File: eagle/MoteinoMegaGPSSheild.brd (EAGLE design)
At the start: 58.1 x 33.6 mm, 32 parts, among them J1 BilgeSwitch, J2 Button, J3 LED, J4 DS18B20, J5 DS18B20, J6 GND, J7 OKI-78SR-5/1.5, J8 5V, J9 12-24V_VCC, Q1 NDP6020P, Q2 IRF9Z14PBF, Q3 2N7000, Q4 IRF9Z14PBF, Q5 2N7000

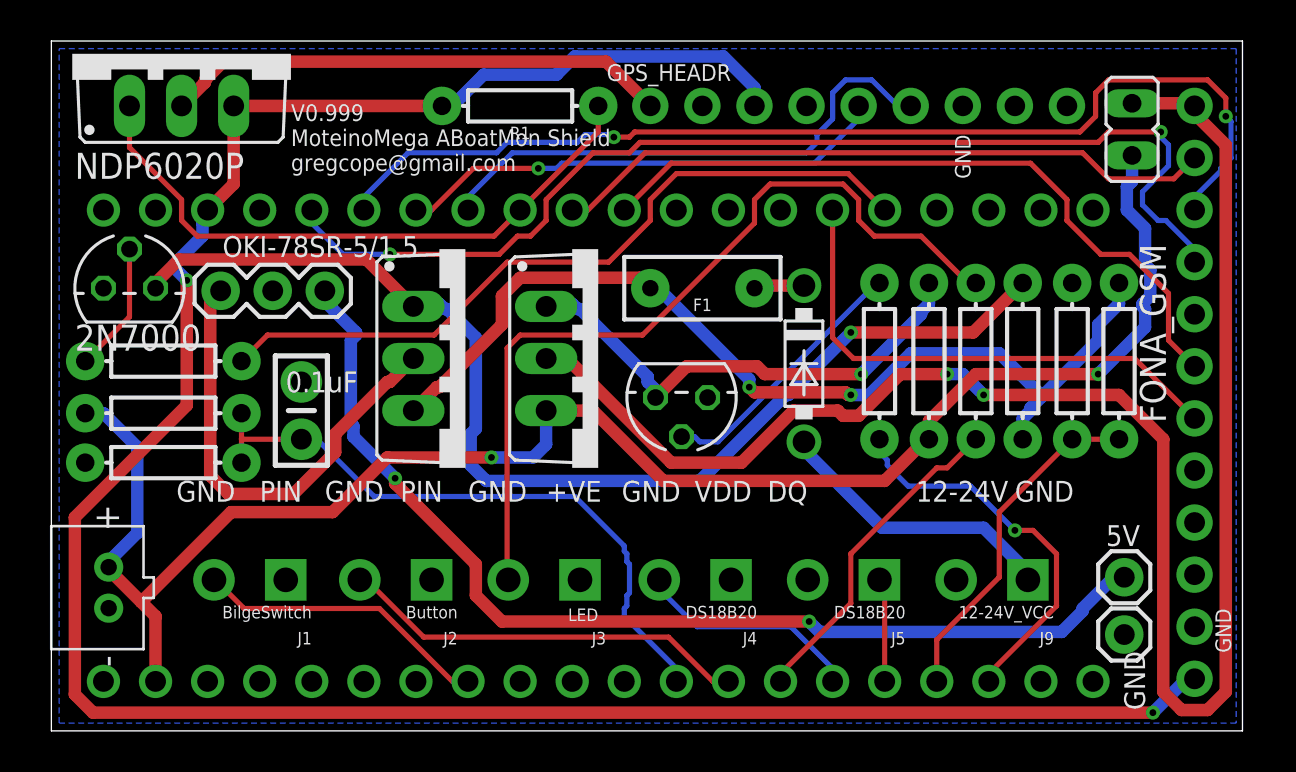
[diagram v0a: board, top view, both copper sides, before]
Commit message: Routed 100%, finally
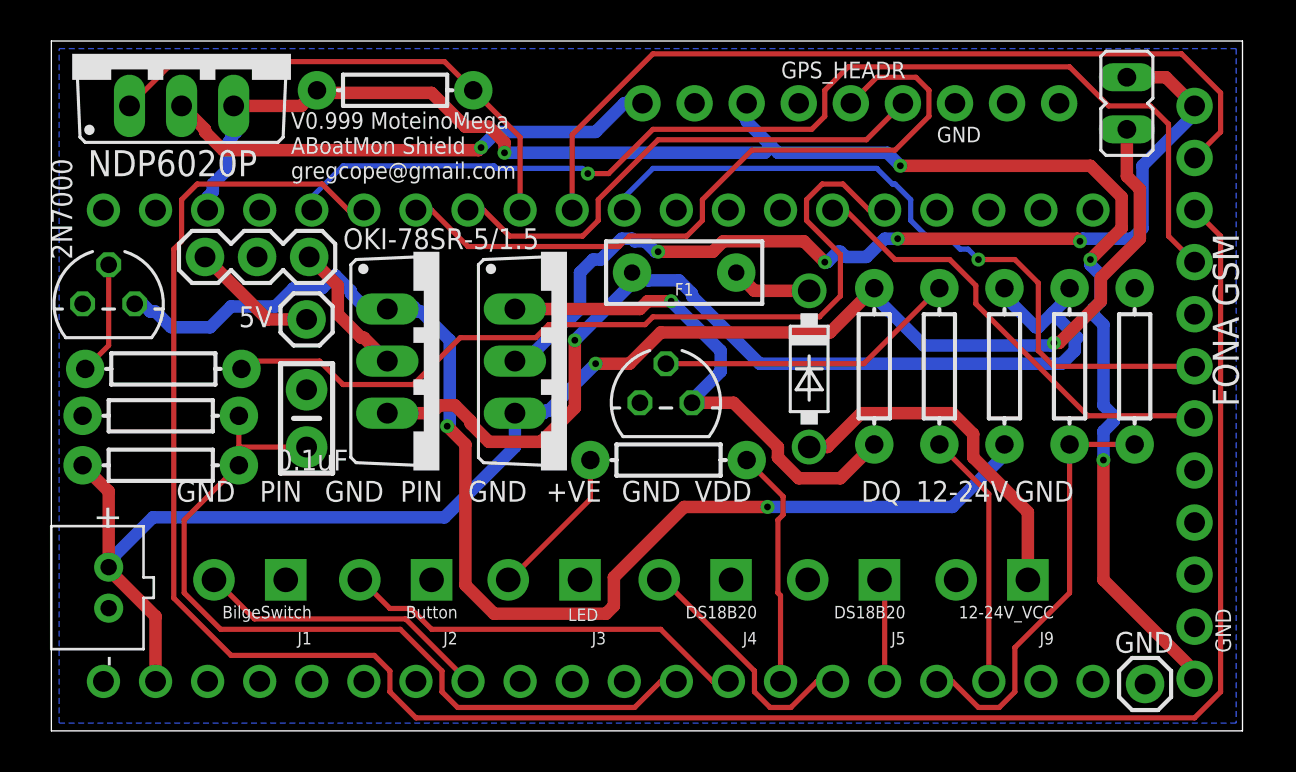
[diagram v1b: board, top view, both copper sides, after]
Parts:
- JP2: value FONA_GSM -> FONA GSM
- moved J8 41.8 mm to (12.4, 49.3)
- moved R7 15.7 mm to (30.1, 42.4), turned to 0 degrees
- moved R1 6.14 mm to (16.8, 60.5)
- moved J7 6.07 mm to (7.49, 52.3), turned to 0 degrees
- moved R6 3.06 mm to (52.8, 47.0)
- moved R10 2.93 mm to (43.3, 47.0)
- moved R8 2.68 mm to (40.1, 47.0), turned to 90 degrees
- moved J6 2.62 mm to (53.3, 31.5)
- moved R2 2.54 mm to (5.33, 42.2)
- moved R5 2.43 mm to (49.7, 47.0)
- moved R3 2.29 mm to (5.33, 44.6)
- moved Q4 1.53 mm to (25.1, 47.2)
- moved JP3 1.30 mm to (52.5, 59.8)
- moved Q2 1.28 mm to (18.9, 47.2)
- moved Q3 1.27 mm to (2.79, 50.0)
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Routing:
- net D9: track 52.5 -> 107.9 mm, vias 2 -> 0
- net 5V_VCC: track 51.7 -> 6.22 mm, vias 2 -> 0
- net JUMPER: track 84.0 -> 46.9 mm, vias 2 -> 4
- net 3.3V: track 116.0 -> 81.7 mm, vias 2 -> 4
- net N$7: track 40.8 -> 7.54 mm
- net 12-24V-SW: track 22.8 -> 6.73 mm
- net D10_RX1: track 24.1 -> 34.8 mm, vias 1 -> 0
- net A0: track 31.1 -> 40.5 mm
- net D13_NETSTAT: track 32.5 -> 41.4 mm
- net N$2: track 55.6 -> 62.1 mm, vias 1 -> 2
- net D30: track 19.1 -> 12.6 mm, vias 1 -> 0
- net D12: track 30.6 -> 25.0 mm
- net VIN: track 84.2 -> 78.8 mm
- net D19_PWRON: track 36.5 -> 41.7 mm
- net D26: track 16.1 -> 11.7 mm
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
